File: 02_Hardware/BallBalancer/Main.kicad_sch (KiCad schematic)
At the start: 59 parts, among them J1 USB_B_Micro, J2 Raspberry PI UART, J3 SWD, J4 Reference switch 1, J5 ENCODER 1, J6 ENCODER 2, J7 Reference switch 2, U1 STM32L412K8Tx, U2 USBLC6-2SC6

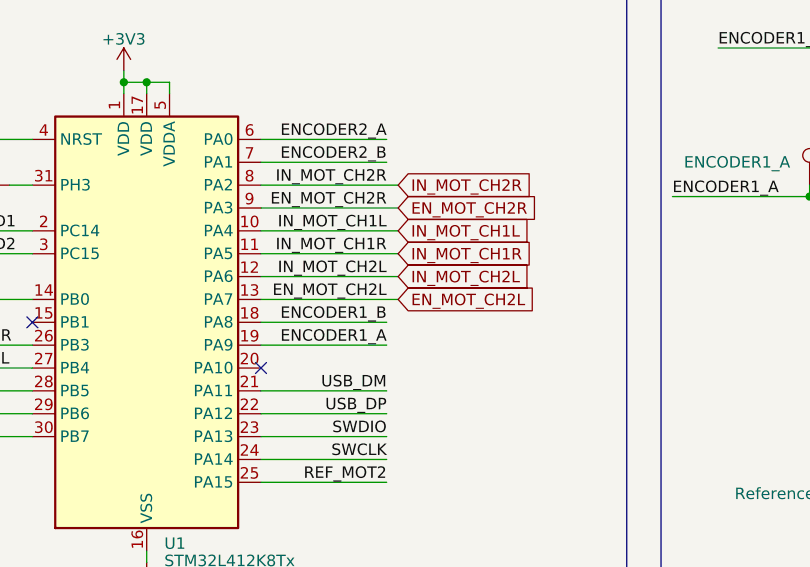
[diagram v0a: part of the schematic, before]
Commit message: CAD files and hardware manufacturing data added
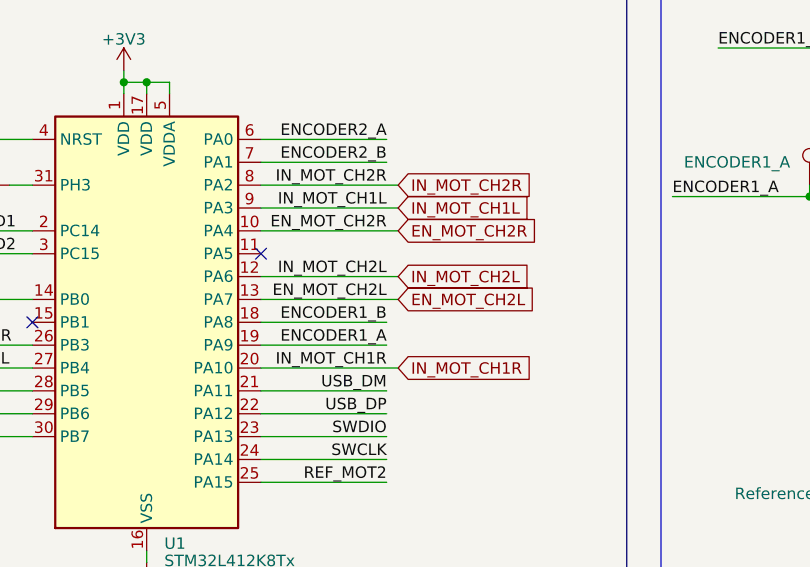
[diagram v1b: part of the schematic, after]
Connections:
- net EN_MOT_CH2R: now also U1.10 (PA4); no longer U1.9 (PA3)
- net IN_MOT_CH1L: now also U1.9 (PA3); no longer U1.10 (PA4)
- net IN_MOT_CH1R: now also U1.20 (PA10); no longer U1.11 (PA5)
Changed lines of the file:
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@@
   (no_connect (at 39.37 170.18))
   (no_connect (at 234.95 38.1))
-  (no_connect (at 80.01 91.44))
+  (no_connect (at 80.01 78.74))
   (wire (pts (xy 130.81 55.88) (xy 157.48 55.88))
     (stroke (width 0) (type default))
@@
     (stroke (width 0) (type default))
   )
+  (wire (pts (xy 80.01 73.66) (xy 95.25 73.66))
+    (stroke (width 0) (type default))
+  )
+  (wire (pts (xy 44.45 71.12) (xy 43.18 71.12))
+    (stroke (width 0) (type default))
+  )
+  (wire (pts (xy 104.14 125.73) (xy 104.14 128.27))
+    (stroke (width 0) (type default))
+  )
+  (wire (pts (xy 160.02 34.29) (xy 181.61 34.29))
+    (stroke (width 0) (type default))
+  )
+  (wire (pts (xy 259.08 132.08) (xy 270.51 132.08))
+    (stroke (width 0) (type default))
+  )
+  (wire (pts (xy 52.07 71.12) (xy 54.61 71.12))
+    (stroke (width 0) (type default))
+  )
+  (wire (pts (xy 157.48 86.36) (xy 157.48 82.55))
+    (stroke (width 0) (type default))
+  )
+  (wire (pts (xy 149.86 72.39) (xy 149.86 74.93))
+    (stroke (width 0) (type default))
+  )
+  (wire (pts (xy 38.1 88.9) (xy 54.61 88.9))
+    (stroke (width 0) (type default))
+  )
+  (wire (pts (xy 156.21 113.03) (xy 154.94 113.03))
+    (stroke (width 0) (type default))
+  )
+  (wire (pts (xy 48.26 170.18) (xy 48.26 171.45))
+    (stroke (width 0) (type default))
+  )
+  (wire (pts (xy 179.07 137.16) (xy 179.07 139.7))
+    (stroke (width 0) (type default))
+  )
+  (wire (pts (xy 80.01 96.52) (xy 93.98 96.52))
+    (stroke (width 0) (type default))
+  )
+  (wire (pts (xy 237.49 57.15) (xy 237.49 55.88))
+    (stroke (width 0) (type default))
+  )
+  (wire (pts (xy 234.95 116.84) (xy 246.38 116.84))
+    (stroke (width 0) (type default))
+  )
+  (wire (pts (xy 220.98 72.39) (xy 207.01 72.39))
+    (stroke (width 0) (type default))
+  )
+  (wire (pts (xy 72.39 26.67) (xy 72.39 27.94))
+    (stroke (width 0) (type default))
+  )
+  (wire (pts (xy 93.98 133.35) (xy 93.98 134.62))
+    (stroke (width 0) (type default))
+  )
+  (wire (pts (xy 99.06 170.18) (xy 107.95 170.18))
+    (stroke (width 0) (type default))
+  )
+  (wire (pts (xy 88.9 30.48) (xy 90.17 30.48))
+    (stroke (width 0) (type default))
+  )
+  (wire (pts (xy 52.07 35.56) (xy 52.07 36.83))
+    (stroke (width 0) (type default))
+  )
+  (wire (pts (xy 80.01 91.44) (xy 95.25 91.44))
+    (stroke (width 0) (type default))
+  )
+  (wire (pts (xy 62.23 25.4) (xy 62.23 26.67))
+    (stroke (width 0) (type default))
+  )
+  (wire (pts (xy 167.64 72.39) (xy 175.26 72.39))
+    (stroke (width 0) (type default))
+  )
+  (wire (pts (xy 67.31 111.76) (xy 67.31 113.03))
+    (stroke (width 0) (type default))
+  )
+  (wire (pts (xy 156.21 109.22) (xy 156.21 113.03))
+    (stroke (width 0) (type default))
+  )
+  (wire (pts (xy 229.87 72.39) (xy 229.87 74.93))
+    (stroke (width 0) (type default))
+  )
+  (wire (pts (xy 80.01 88.9) (xy 93.98 88.9))
+    (stroke (width 0) (type default))
+  )
+  (wire (pts (xy 110.49 33.02) (xy 102.87 33.02))
+    (stroke (width 0) (type default))
+  )
+  (wire (pts (xy 62.23 35.56) (xy 62.23 36.83))
+    (stroke (width 0) (type default))
+  )
   (wire (pts (xy 80.01 76.2) (xy 95.25 76.2))
     (stroke (width 0) (type default))
   )
-  (wire (pts (xy 44.45 71.12) (xy 43.18 71.12))
-    (stroke (width 0) (type default))
-  )
-  (wire (pts (xy 104.14 125.73) (xy 104.14 128.27))
-    (stroke (width 0) (type default))
-  )
-  (wire (pts (xy 160.02 34.29) (xy 181.61 34.29))
-    (stroke (width 0) (type default))
-  )
-  (wire (pts (xy 259.08 132.08) (xy 270.51 132.08))
-    (stroke (width 0) (type default))
-  )
-  (wire (pts (xy 52.07 71.12) (xy 54.61 71.12))
-    (stroke (width 0) (type default))
-  )
-  (wire (pts (xy 157.48 86.36) (xy 157.48 82.55))
-    (stroke (width 0) (type default))
-  )
-  (wire (pts (xy 149.86 72.39) (xy 149.86 74.93))
-    (stroke (width 0) (type default))
-  )
-  (wire (pts (xy 38.1 88.9) (xy 54.61 88.9))
-    (stroke (width 0) (type default))
-  )
-  (wire (pts (xy 156.21 113.03) (xy 154.94 113.03))
-    (stroke (width 0) (type default))
-  )
-  (wire (pts (xy 48.26 170.18) (xy 48.26 171.45))
-    (stroke (width 0) (type default))
-  )
-  (wire (pts (xy 179.07 137.16) (xy 179.07 139.7))
-    (stroke (width 0) (type default))
-  )
-  (wire (pts (xy 80.01 96.52) (xy 93.98 96.52))
-    (stroke (width 0) (type default))
-  )
-  (wire (pts (xy 237.49 57.15) (xy 237.49 55.88))
-    (stroke (width 0) (type default))
-  )
-  (wire (pts (xy 234.95 116.84) (xy 246.38 116.84))
-    (stroke (width 0) (type default))
-  )
-  (wire (pts (xy 220.98 72.39) (xy 207.01 72.39))
-    (stroke (width 0) (type default))
-  )
-  (wire (pts (xy 72.39 26.67) (xy 72.39 27.94))
-    (stroke (width 0) (type default))
-  )
-  (wire (pts (xy 93.98 133.35) (xy 93.98 134.62))
-    (stroke (width 0) (type default))
-  )
-  (wire (pts (xy 99.06 170.18) (xy 107.95 170.18))
-    (stroke (width 0) (type default))
-  )
-  (wire (pts (xy 88.9 30.48) (xy 90.17 30.48))
-    (stroke (width 0) (type default))
-  )
-  (wire (pts (xy 52.07 35.56) (xy 52.07 36.83))
-    (stroke (width 0) (type default))
-  )
-  (wire (pts (xy 80.01 78.74) (xy 95.25 78.74))
-    (stroke (width 0) (type default))
-  )
-  (wire (pts (xy 62.23 25.4) (xy 62.23 26.67))
-    (stroke (width 0) (type default))
-  )
-  (wire (pts (xy 167.64 72.39) (xy 175.26 72.39))
-    (stroke (width 0) (type default))
-  )
-  (wire (pts (xy 67.31 111.76) (xy 67.31 113.03))
-    (stroke (width 0) (type default))
-  )
-  (wire (pts (xy 156.21 109.22) (xy 156.21 113.03))
-    (stroke (width 0) (type default))
-  )
-  (wire (pts (xy 229.87 72.39) (xy 229.87 74.93))
-    (stroke (width 0) (type default))
-  )
-  (wire (pts (xy 80.01 88.9) (xy 93.98 88.9))
-    (stroke (width 0) (type default))
-  )
-  (wire (pts (xy 110.49 33.02) (xy 102.87 33.02))
-    (stroke (width 0) (type default))
-  )
-  (wire (pts (xy 62.23 35.56) (xy 62.23 36.83))
-    (stroke (width 0) (type default))
-  )
-  (wire (pts (xy 80.01 73.66) (xy 95.25 73.66))
-    (stroke (width 0) (type default))
-  )
   (wire (pts (xy 44.45 113.03) (xy 46.99 113.03))
     (stroke (width 0) (type default))
@@
     (effects (font (size 1.27 1.27)) (justify right bottom))
   )
-  (label "IN_MOT_CH1L" (at 93.98 76.2 180) (fields_autoplaced)
+  (label "IN_MOT_CH1L" (at 93.98 73.66 180) (fields_autoplaced)
     (effects (font (size 1.27 1.27)) (justify right bottom))
   )
@@
     (effects (font (size 1.27 1.27)) (justify right bottom))
   )
-  (label "EN_MOT_CH2R" (at 93.98 73.66 180) (fields_autoplaced)
+  (label "EN_MOT_CH2R" (at 93.98 76.2 180) (fields_autoplaced)
     (effects (font (size 1.27 1.27)) (justify right bottom))
   )
@@
     (effects (font (size 1.27 1.27)) (justify right bottom))
   )
-  (label "IN_MOT_CH1R" (at 93.98 78.74 180) (fields_autoplaced)
+  (label "IN_MOT_CH1R" (at 93.98 91.44 180) (fields_autoplaced)
     (effects (font (size 1.27 1.27)) (justify right bottom))
   )
@@
     )
   )
-  (global_label "EN_MOT_CH2R" (shape input) (at 95.25 73.66 0) (fields_autoplaced)
+  (global_label "EN_MOT_CH2R" (shape input) (at 95.25 76.2 0) (fields_autoplaced)
     (effects (font (size 1.27 1.27)) (justify left))
-    (property "Intersheetrefs" "${INTERSHEET_REFS}" (at 111.4 73.66 0)
+    (property "Intersheetrefs" "${INTERSHEET_REFS}" (at 111.4 76.2 0)
       (effects (font (size 1.27 1.27)) (justify left) hide)
     )
@@
     )
   )
-  (global_label "IN_MOT_CH1R" (shape input) (at 95.25 78.74 0) (fields_autoplaced)
+  (global_label "IN_MOT_CH1R" (shape input) (at 95.25 91.44 0) (fields_autoplaced)
     (effects (font (size 1.27 1.27)) (justify left))
-    (property "Intersheetrefs" "${INTERSHEET_REFS}" (at 110.8558 78.74 0)
+    (property "Intersheetrefs" "${INTERSHEET_REFS}" (at 110.8558 91.44 0)
       (effects (font (size 1.27 1.27)) (justify left) hide)
     )
@@
     )
   )
-  (global_label "IN_MOT_CH1L" (shape input) (at 95.25 76.2 0) (fields_autoplaced)
+  (global_label "IN_MOT_CH1L" (shape input) (at 95.25 73.66 0) (fields_autoplaced)
     (effects (font (size 1.27 1.27)) (justify left))
-    (property "Intersheetrefs" "${INTERSHEET_REFS}" (at 110.6139 76.2 0)
+    (property "Intersheetrefs" "${INTERSHEET_REFS}" (at 110.6139 73.66 0)
       (effects (font (size 1.27 1.27)) (justify left) hide)
     )
